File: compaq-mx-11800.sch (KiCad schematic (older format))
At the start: 252 parts, among them J1 Conn_01x16_Female, J2 Conn_01x16_Female, j1 MX-NoLED, k1 MX-NoLED, m1 MX-NoLED, p1 MX-NoLED, q1 MX-NoLED, t1 MX-NoLED, u1 MX-NoLED, x1 MX-NoLED, y1 MX-NoLED

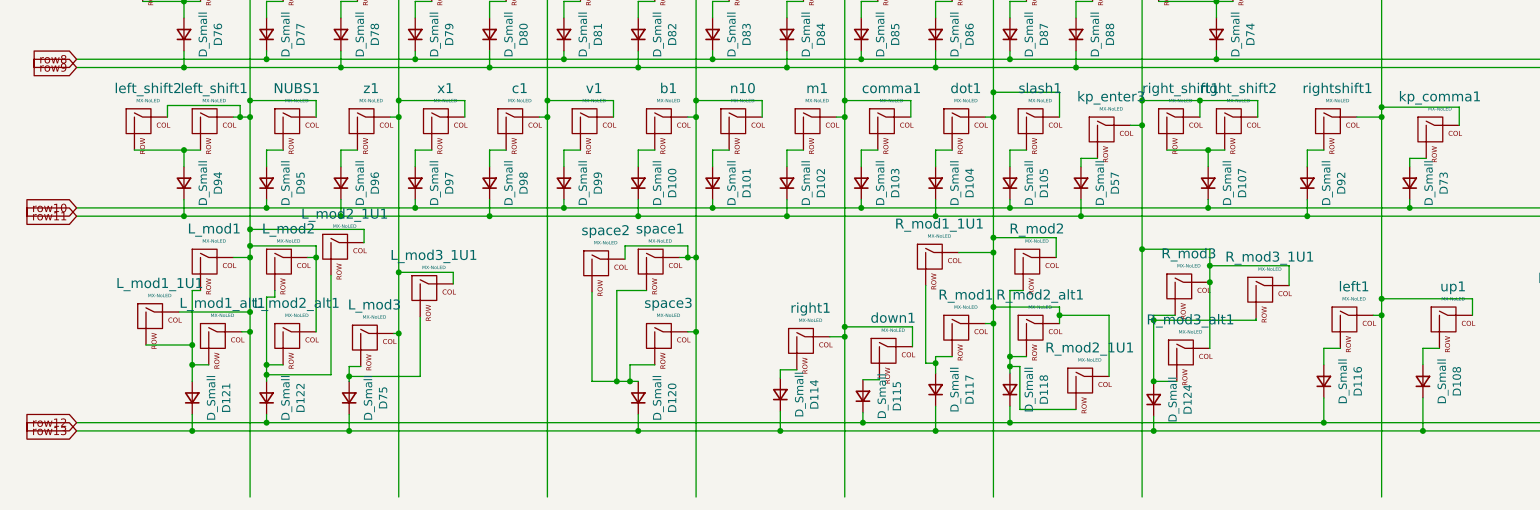
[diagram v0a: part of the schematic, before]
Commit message: clean up schematics
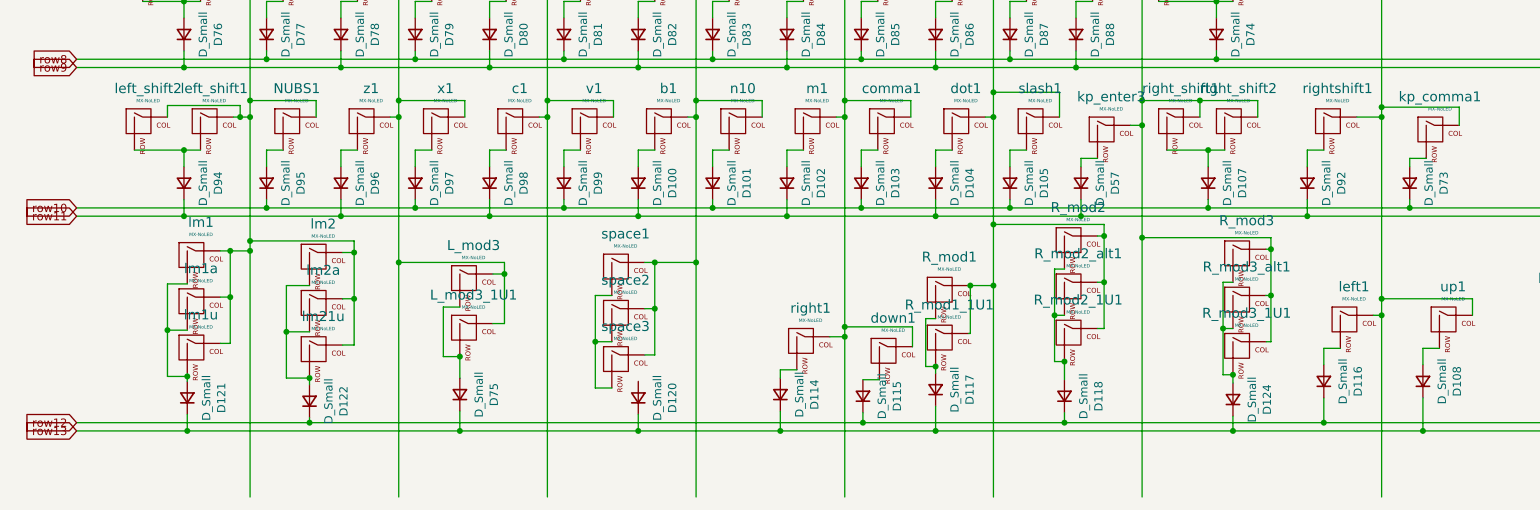
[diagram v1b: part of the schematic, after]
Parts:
- renumbered L_mod1 to lm1, L_mod1_alt1 to lm1a, L_mod1_1U1 to lm1u, L_mod2 to lm2, L_mod2_1U1 to lm21u, L_mod2_alt1 to lm2a
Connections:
- wire segments 832 -> 823
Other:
- moved on the sheet: D118, D121, D122, D124, D75, L_mod3, L_mod3_1U1, R_mod1, R_mod1_1U1, R_mod2, R_mod2_1U1, R_mod2_alt1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
